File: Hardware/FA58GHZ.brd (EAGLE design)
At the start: 81.3 x 34.3 mm, 16 parts, among them U1 ATMEGA328P_TQFP, Y1 16MHZ

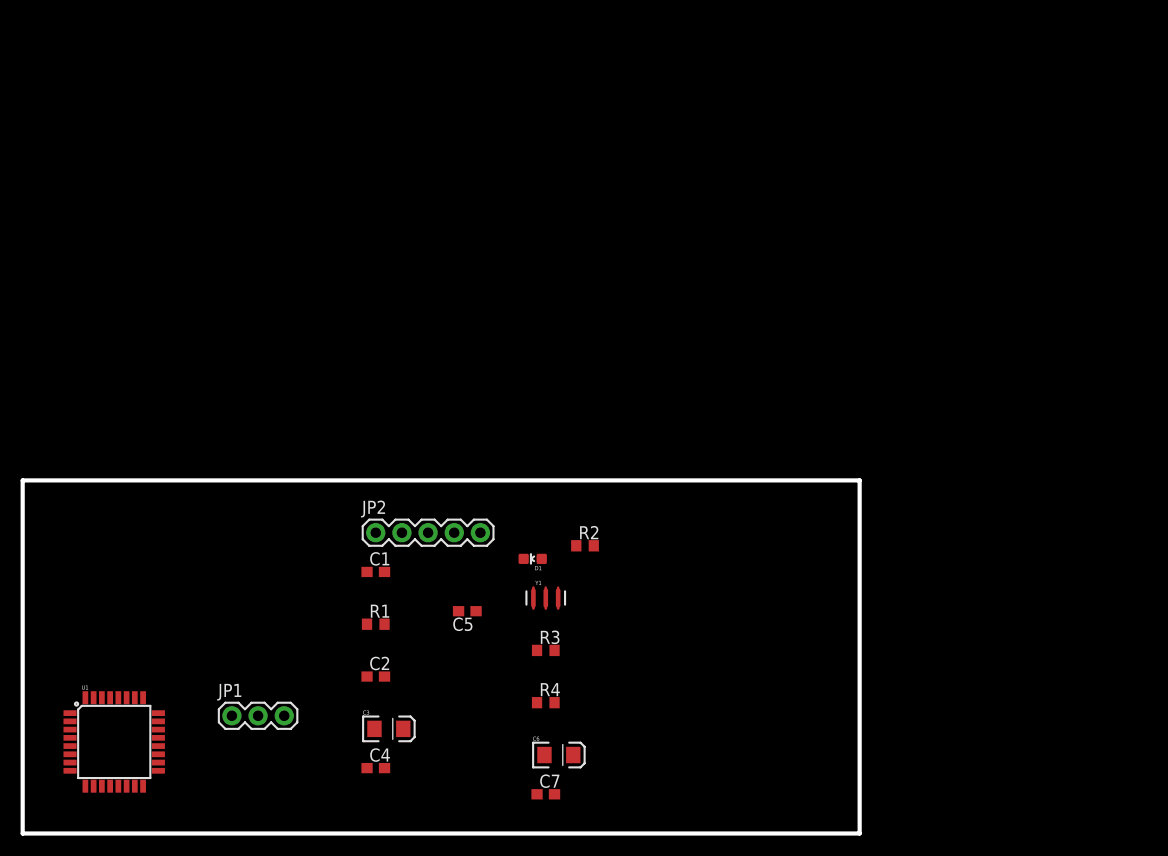
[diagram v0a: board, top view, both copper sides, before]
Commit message: Backup: Working in the Schematic, Footprints and PCB
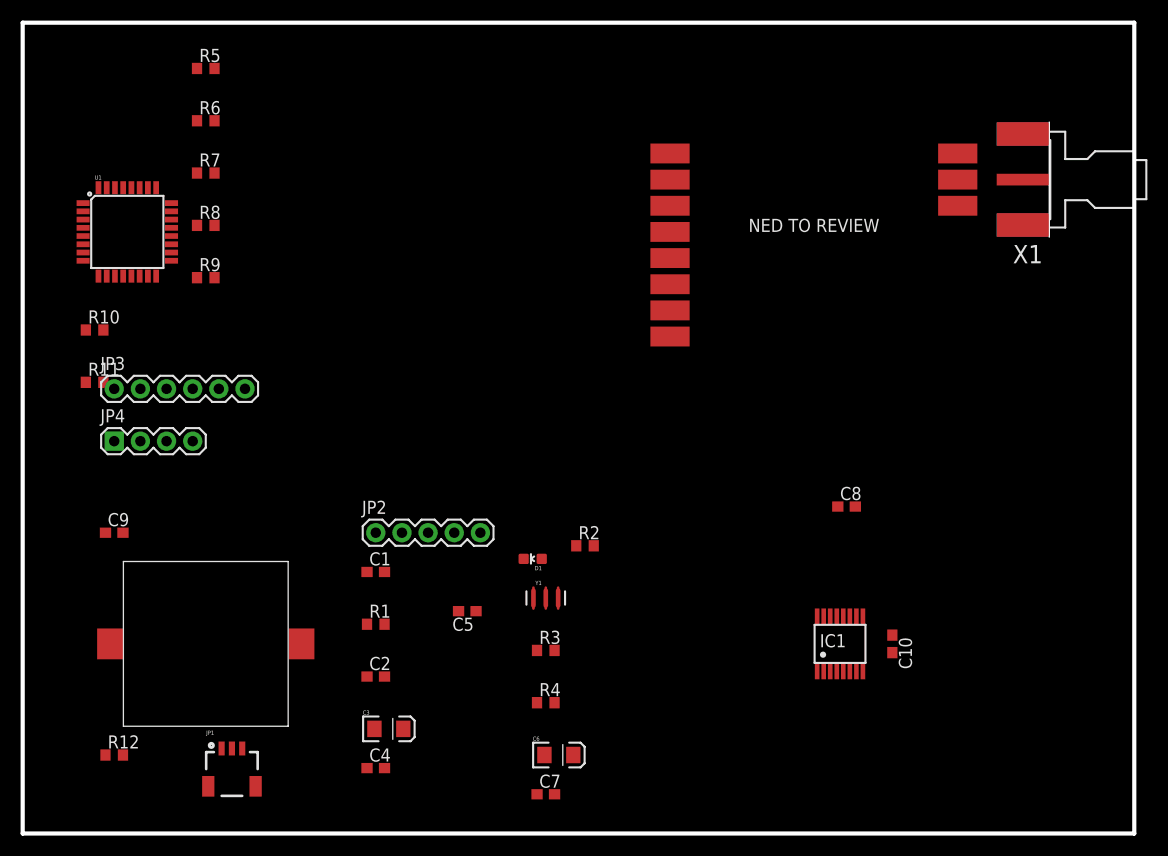
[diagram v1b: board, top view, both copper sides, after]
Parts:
- added C10, C8, C9: 0.1uF, resistor:C0603
- added IC1: MAX4311EEE, maxim:QSOP16
- added JP3: (no value), SparkFun-Connectors:1X06
- added JP4: (no value), SparkFun-Connectors:1X04
- added R10, R11, R12: 1k, resistor:R0603
- added R5, R6, R7: 10k, resistor:R0603
- added R8: 470, resistor:R0603
- added R9: 5k1, resistor:R0603
- added SG1: BUZZERSMD, SparkFun-Electromechanical:BUZZER-CMT1603
- added U2: RX5808, FreakyAttic-EagleLibrary:RX5808
- added X1: SMA, con-coax:J502-ND-142-0701-881/886
- JP1: device SparkFun-Connectors:1X03 -> SparkFun-Connectors:1X03-1MM-RA
- R3, R4: value 10k -> ?
- moved U1 49.5 mm to (10.2, 58.4)
- moved JP1 3.17 mm to (20.3, 8.26)
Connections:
- net N$6 renamed LED
- new net BUT1: U1.32
- new net BUT2: U1.1
- new net CH1: R7.1, U1.14
- new net CH2: R5.1, U1.15
- new net CH3: R6.1, U1.16
- new net N$10: R12.1, U1.9
- new net N$11: SG1.P$2, U1.10
- new net N$12: R12.2, SG1.P$1
- new net N$13: R6.2, U2.P$9
- new net N$14: R5.2, U2.P$8
- new net N$15: R7.2, U2.P$7
- new net N$16: U2.P$11, X1.1
- new net N$6: R8.1, U1.11
- new net N$7: R9.1, U1.13
- new net N$8: R10.1, U1.30
- new net N$9: R11.1, U1.31
- new net OSD: IC1.5, R8.2, R9.2
- new net RSSI1: JP4.2, U1.19, U2.P$4
- new net RSSI2: JP4.4, U1.22
- new net SEL0: IC1.2
- new net SEL1: IC1.1
- new net VIDEO1: IC1.7, JP3.2, U2.P$2
- new net VIDEO2: IC1.10, JP3.4
- new net VIDEO3: IC1.12, JP3.6
- new net VIDEO_OUT: IC1.15, IC1.16
- net AN_VPOW: now also C9.2
- net GND: now also C10.1, C8.2, C9.1, IC1.13, JP3.1, JP3.3, JP3.5, JP4.1, JP4.3, U2.P$1, U2.P$10, U2.P$12, U2.P$6, X1.G@1, X1.G@2, X1.G@3, X1.G@4
- net VCC: now also C10.2, C8.1, IC1.14, IC1.4, U2.P$5
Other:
- board size 81.3 x 34.3 mm -> 108 x 78.7 mm
